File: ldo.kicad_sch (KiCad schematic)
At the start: 3 parts, among them IC4 LDO

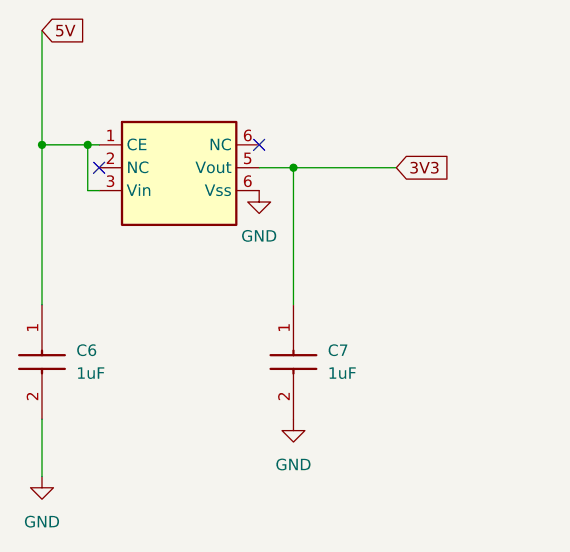
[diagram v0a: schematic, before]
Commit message: initial PCB draft!
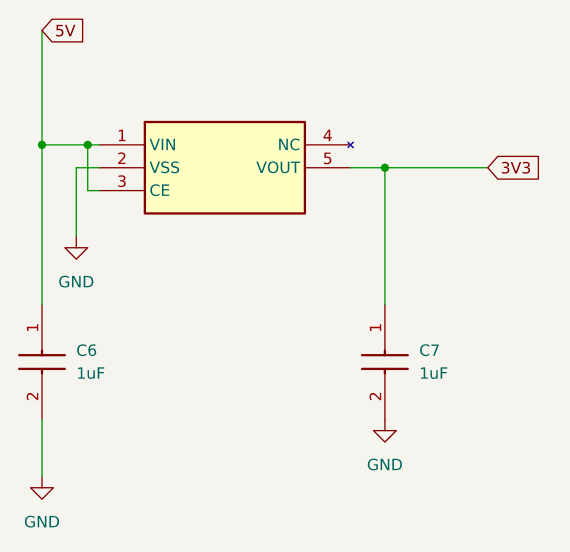
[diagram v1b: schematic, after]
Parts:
- IC4: footprint (none) -> group127:LDO; symbol group127:XC6210A332MR-G -> group127:LDO; Height (none) -> 1.3; Manufacturer_Name (none) -> Torex; Manufacturer_Part_Number (none) -> XC6210A332MR-G; Mouser Part Number (none) -> 865-XC6210A332MR-G; Mouser Price/Stock (none) -> https://www.mouser.co.uk/ProductDetail/Torex-Semiconductor/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
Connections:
- net GND: now also IC4.2 (VSS); no longer IC4.6 (Vss)
- no-connect marks 2 -> 0
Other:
- moved on the sheet: C7
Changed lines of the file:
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@@
 	)
 	(junction
-		(at 179.07 82.55)
+		(at 189.23 82.55)
 		(diameter 0)
 		(color 0 0 0 0)
@@
 		(color 0 0 0 0)
 	)
-	(no_connect
-		(at 157.48 82.55)
-	)
-	(no_connect
-		(at 175.26 80.01)
+	(wire
+		(pts
+			(xy 157.48 82.55) (xy 154.94 82.55)
+		)
+		(stroke
+			(width 0)
+			(type default)
+		)
 	)
 	(wire
@@
 	(wire
 		(pts
-			(xy 179.07 82.55) (xy 179.07 97.79)
-		)
-		(stroke
-			(width 0)
-			(type default)
-		)
-	)
-	(wire
-		(pts
-			(xy 179.07 82.55) (xy 190.5 82.55)
+			(xy 189.23 82.55) (xy 189.23 97.79)
+		)
+		(stroke
+			(width 0)
+			(type default)
+		)
+	)
+	(wire
+		(pts
+			(xy 189.23 82.55) (xy 200.66 82.55)
 		)
 		(stroke
@@
 	(wire
 		(pts
-			(xy 175.26 82.55) (xy 179.07 82.55)
+			(xy 185.42 82.55) (xy 189.23 82.55)
 		)
 		(stroke
@@
 		(pts
 			(xy 151.13 80.01) (xy 151.13 97.79)
+		)
+		(stroke
+			(width 0)
+			(type default)
+		)
+	)
+	(wire
+		(pts
+			(xy 154.94 82.55) (xy 154.94 90.17)
 		)
 		(stroke
@@
 	(global_label "3V3"
 		(shape input)
-		(at 190.5 82.55 0)
+		(at 200.66 82.55 0)
 		(fields_autoplaced yes)
 		(effects
@@
 		)
 		(property "Intersheetrefs" "${INTERSHEET_REFS}"
-			(at 196.9928 82.55 0)
+			(at 207.1528 82.55 0)
 			(effects
 				(font
@@
 	(symbol
 		(lib_id "power:GND")
-		(at 179.07 110.49 0)
+		(at 189.23 110.49 0)
 		(unit 1)
 		(exclude_from_sim no)
@@
 		(fields_autoplaced yes)
 		(property "Reference" "#PWR020"
-			(at 179.07 116.84 0)
+			(at 189.23 116.84 0)
 			(effects
 				(font
@@
 		)
 		(property "Value" "GND"
-			(at 179.07 115.57 0)
+			(at 189.23 115.57 0)
 			(effects
 				(font
@@
 		)
 		(property "Footprint" ""
-			(at 179.07 110.49 0)
+			(at 189.23 110.49 0)
 			(effects
 				(font
@@
 		)
 		(property "Datasheet" ""
-			(at 179.07 110.49 0)
+			(at 189.23 110.49 0)
 			(effects
 				(font
@@
 		)
 		(property "Description" "Power symbol creates a global label with name \"GND\" , ground"
-			(at 179.07 110.49 0)
+			(at 189.23 110.49 0)
 			(effects
 				(font
@@
 	(symbol
 		(lib_id "group127:0805Capacitor")
-		(at 179.07 97.79 270)
+		(at 189.23 97.79 270)
 		(unit 1)
 		(exclude_from_sim no)
@@
 		(fields_autoplaced yes)
 		(property "Reference" "C7"
-			(at 182.88 102.8699 90)
+			(at 193.04 102.8699 90)
 			(effects
 				(font
@@
 		)
 		(property "Value" "1uF"
-			(at 182.88 105.4099 90)
+			(at 193.04 105.4099 90)
 			(effects
 				(font
@@
 		)
 		(property "Footprint" "Capacitor_SMD:C_0805_2012Metric"
-			(at 82.88 106.68 0)
+			(at 93.04 106.68 0)
 			(effects
 				(font
@@
 		)
 		(property "Datasheet" "http://datasheets.avx.com/X7RDielectric.pdf"
-			(at -17.12 106.68 0)
+			(at -6.96 106.68 0)
 			(effects
 				(font
@@
 		)
 		(property "Description" "0805 X7R ceramic capacitor,100nF 50V AVX 0805 Standard 100nF Ceramic Multilayer Capacitor, 50 V dc, +125degC, X7R Dielectric,  /-10% SMD"
-			(at 179.07 97.79 0)
+			(at 189.23 97.79 0)
 			(effects
 				(font
@@
 		)
 		(property "Height" "0.94"
-			(at -217.12 106.68 0)
+			(at -206.96 106.68 0)
 			(effects
 				(font
@@
 		)
 		(property "Mouser Part Number" "581-08055C104K"
-			(at -317.12 106.68 0)
+			(at -306.96 106.68 0)
 			(effects
 				(font
@@
 		)
 		(property "Mouser Price/Stock" "https://www.mouser.co.uk/ProductDetail/KYOCERA-AVX/08055C104KAT2A?qs=2ujN4bDBNE9mJvapP%252BjopA%3D%3D"
-			(at -417.12 106.68 0)
+			(at -406.96 106.68 0)
 			(effects
 				(font
@@
 		)
 		(property "Manufacturer_Name" "Kyocera AVX"
-			(at -517.12 106.68 0)
+			(at -506.96 106.68 0)
 			(effects
 				(font
@@
 		)
 		(property "Manufacturer_Part_Number" "08055C104KAT2A"
-			(at -617.12 106.68 0)
+			(at -606.96 106.68 0)
 			(effects
 				(font
@@
 	)
 	(symbol
-		(lib_id "group127:XC6210A332MR-G")
-		(at 166.37 82.55 0)
+		(lib_id "group127:LDO")
+		(at 157.48 80.01 0)
 		(unit 1)
 		(exclude_from_sim no)
@@
 		(fields_autoplaced yes)
 		(property "Reference" "IC4"
-			(at 166.116 75.184 0)
+			(at 157.226 72.644 0)
 			(effects
 				(font
@@
 		)
 		(property "Value" "LDO"
-			(at 172.72 76.2 0)
-			(effects
-				(font
-					(size 1.27 1.27)
-				)
-				(hide yes)
-			)
-		)
-		(property "Footprint" ""
-			(at 167.132 68.834 0)
-			(effects
-				(font
-					(size 1.27 1.27)
-				)
-				(hide yes)
-			)
-		)
-		(property "Datasheet" "https://www.mouser.com/datasheet/2/760/xc6210-3371396.pdf"
-			(at 165.1 63.5 0)
-			(effects
-				(font
-					(size 1.27 1.27)
-				)
+			(at 163.83 73.66 0)
+			(effects
+				(font
+					(size 1.27 1.27)
+				)
+				(hide yes)
+			)
+		)
+		(property "Footprint" "group127:LDO"
+			(at 181.61 174.93 0)
+			(effects
+				(font
+					(size 1.27 1.27)
+				)
+				(justify left top)
+				(hide yes)
+			)
+		)
+		(property "Datasheet" "https://www.torexsemi.com/file/xc6210/XC6210.pdf"
+			(at 181.61 274.93 0)
+			(effects
+				(font
+					(size 1.27 1.27)
+				)
+				(justify left top)
 				(hide yes)
 			)
 		)
 		(property "Description" "LDO Voltage Regulators 700mA High Speed LDO Regulator"
-			(at 165.608 102.87 0)
-			(effects
-				(font
-					(size 1.27 1.27)
-				)
-				(hide yes)
-			)
-		)
-		(pin "6"
-		)
-		(pin "6"
+			(at 157.48 80.01 0)
+			(effects
+				(font
+					(size 1.27 1.27)
+				)
+				(hide yes)
+			)
+		)
+		(property "Height" "1.3"
+			(at 181.61 474.93 0)
+			(effects
+				(font
+					(size 1.27 1.27)
+				)
+				(justify left top)
+				(hide yes)
+			)
+		)
+		(property "Mouser Part Number" "865-XC6210A332MR-G"
+			(at 181.61 574.93 0)
+			(effects
+				(font
+					(size 1.27 1.27)
+				)
+				(justify left top)
+				(hide yes)
+			)
+		)
+		(property "Mouser Price/Stock" "https://www.mouser.co.uk/ProductDetail/Torex-Semiconductor/XC6210A332MR-G?qs=AsjdqWjXhJ%252BGZM2kyDkSFw%3D%3D"
+			(at 181.61 674.93 0)
+			(effects
+				(font
+					(size 1.27 1.27)
+				)
+				(justify left top)
+				(hide yes)
+			)
+		)
+		(property "Manufacturer_Name" "Torex"
+			(at 181.61 774.93 0)
+			(effects
+				(font
+					(size 1.27 1.27)
+				)
+				(justify left top)
+				(hide yes)
+			)
+		)
+		(property "Manufacturer_Part_Number" "XC6210A332MR-G"
+			(at 181.61 874.93 0)
+			(effects
+				(font
+					(size 1.27 1.27)
+				)
+				(justify left top)
+				(hide yes)
+			)
+		)
+		(pin "4"
 		)
 		(pin "2"
@@
 	(symbol
 		(lib_id "power:GND")
-		(at 175.26 85.09 0)
+		(at 154.94 90.17 0)
 		(unit 1)
 		(exclude_from_sim no)
@@
 		(dnp no)
 		(fields_autoplaced yes)
-		(property "Reference" "#PWR019"
-			(at 175.26 91.44 0)
+		(property "Reference" "#PWR034"
+			(at 154.94 96.52 0)
 			(effects
 				(font
@@
 		)
 		(property "Value" "GND"
-			(at 175.26 90.17 0)
+			(at 154.94 95.25 0)
 			(effects
 				(font
@@
 		)
 		(property "Footprint" ""
-			(at 175.26 85.09 0)
+			(at 154.94 90.17 0)
 			(effects
 				(font
@@
 		)
 		(property "Datasheet" ""
-			(at 175.26 85.09 0)
+			(at 154.94 90.17 0)
 			(effects
 				(font
@@
 		)
 		(property "Description" "Power symbol creates a global label with name \"GND\" , ground"
-			(at 175.26 85.09 0)
+			(at 154.94 90.17 0)
 			(effects
 				(font
@@
 			(project "harm_drone"
 				(path "/5ce3566e-4e0f-420e-9b0d-3952cd3c63fd/06c65770-b1a9-4683-9717-b848c80eccc4"
-					(reference "#PWR019")
-					(unit 1)
-				)
-			)
-			(project "ldo"
-				(path "/8c89e2c6-3a4c-42d5-9469-c7cf807a96d1"
-					(reference "#PWR03")
-					(unit 1)
-				)
+					(reference "#PWR034")
+					(unit 1)
+				)
